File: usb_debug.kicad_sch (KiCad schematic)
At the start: 12 parts, among them J10 DBG pads (SWCLK SWDIO GND), J4 USB_C_PROGRAM_POWER

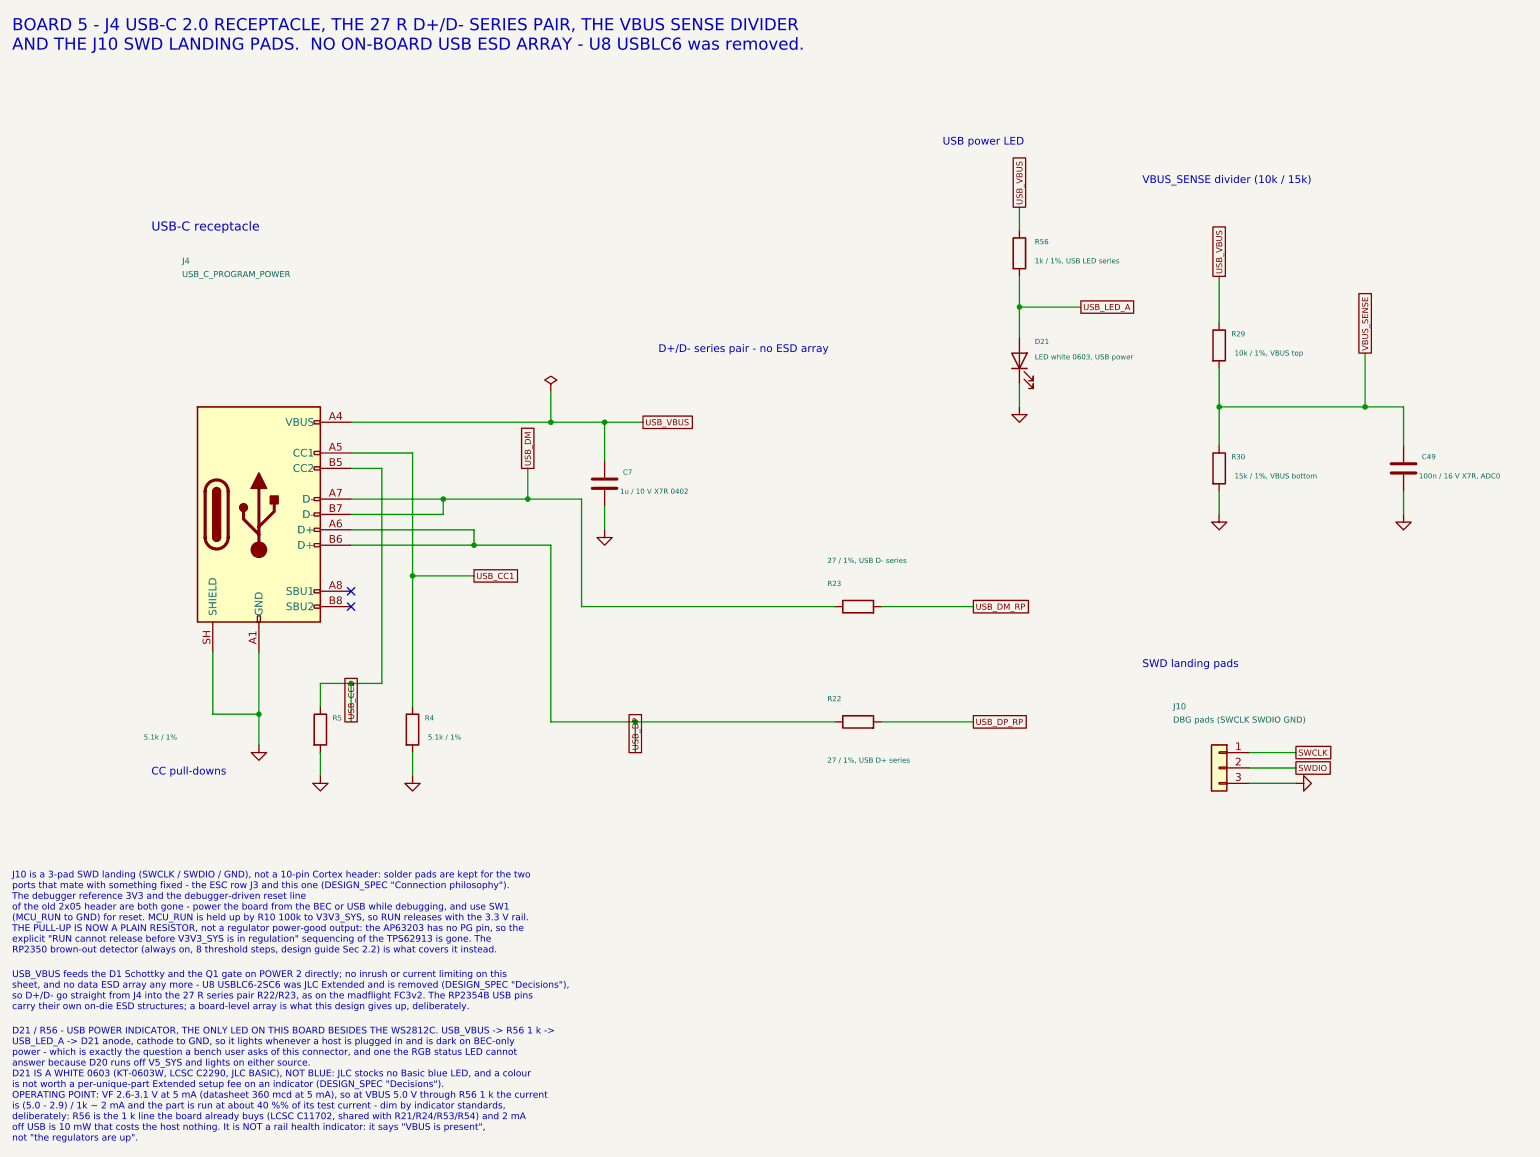
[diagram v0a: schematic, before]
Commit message: update
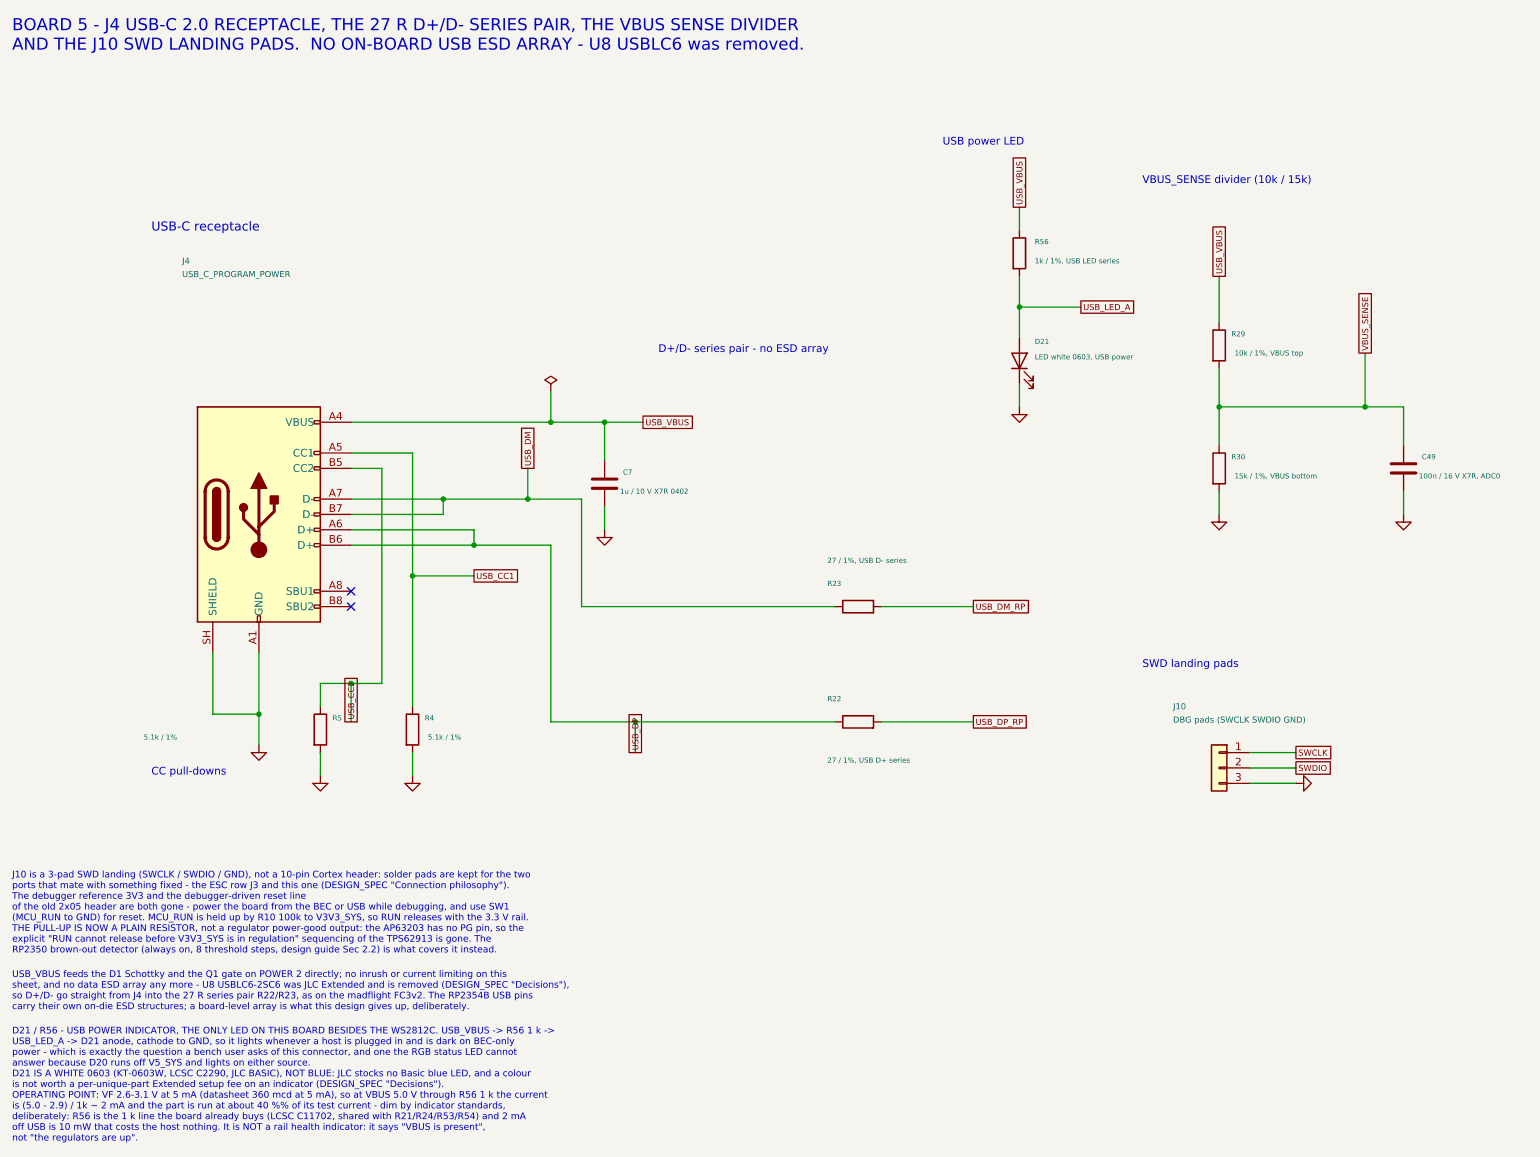
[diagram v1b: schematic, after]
